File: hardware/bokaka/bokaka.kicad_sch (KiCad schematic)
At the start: 0 parts

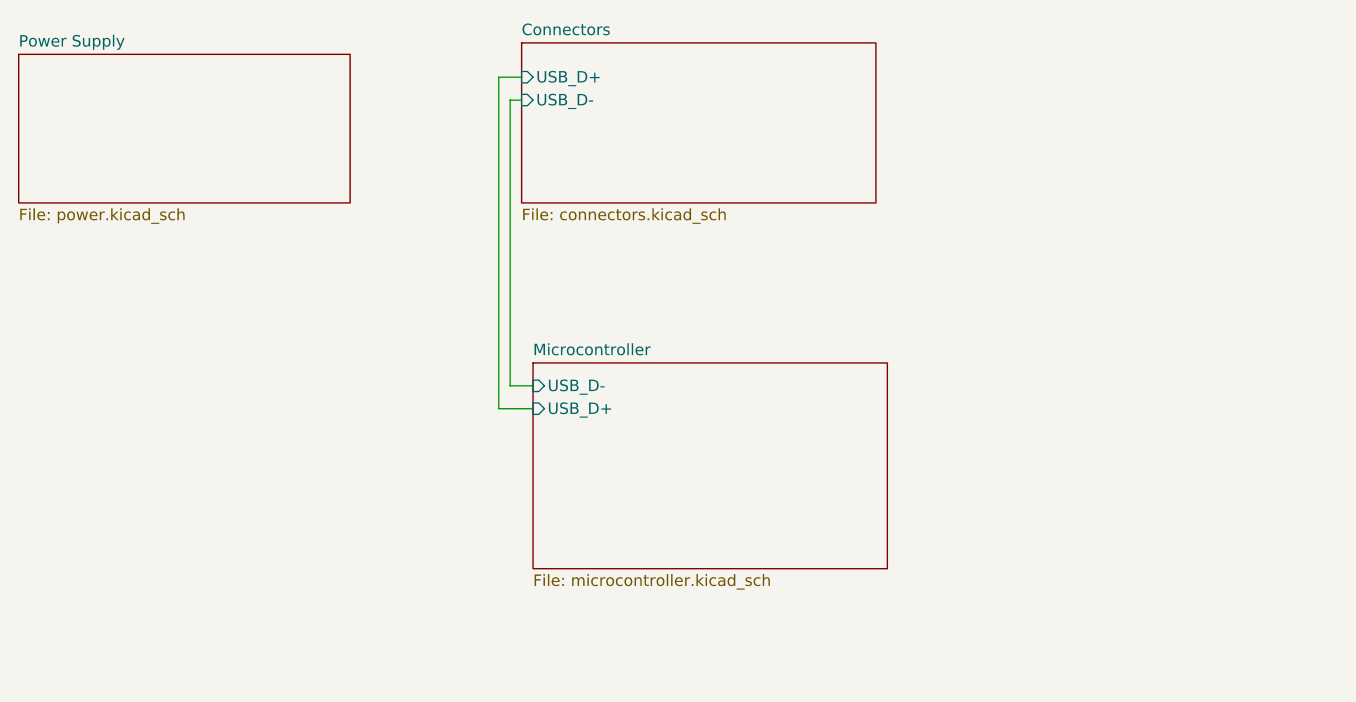
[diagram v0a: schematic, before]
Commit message: Adding rest of design and pdf
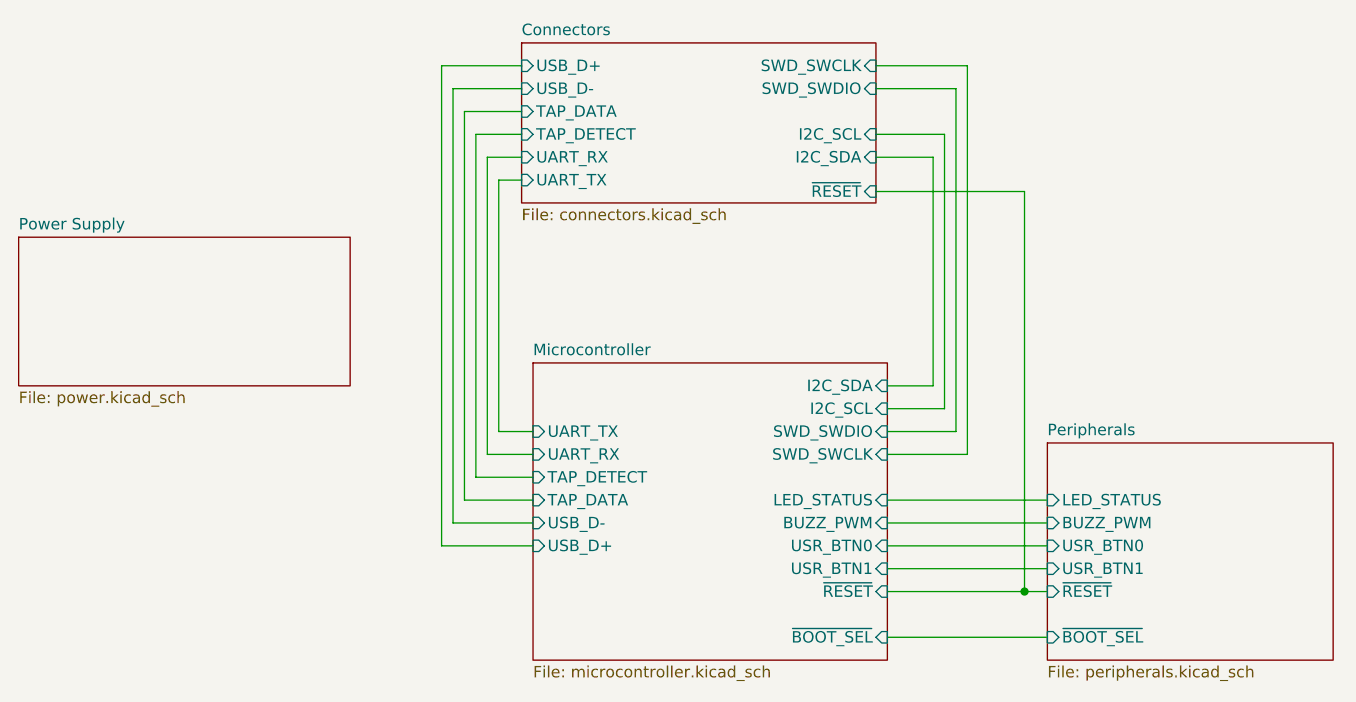
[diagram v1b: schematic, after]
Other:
- added sheet Peripherals (peripherals.kicad_sch)
- sheet Connectors ports: added I2C_SCL, I2C_SDA, SWD_SWCLK, SWD_SWDIO, TAP_DATA, TAP_DETECT, UART_RX, UART_TX, ~{RESET}; removed none
- sheet Microcontroller ports: added BUZZ_PWM, I2C_SCL, I2C_SDA, LED_STATUS, SWD_SWCLK, SWD_SWDIO, TAP_DATA, TAP_DETECT, UART_RX, UART_TX, USR_BTN0, USR_BTN1, ~{BOOT_SEL}, ~{RESET}; removed none
